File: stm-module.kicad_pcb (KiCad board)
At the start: 2 copper layers, 39.3 x 56.1 mm, 25 parts, among them J1 Conn_01x05_Pin, J2 connectorL, J3 connectorR, J4 power, SW1 Reset, U1 STM32G474RETx, U2 TPS7A20xxxDBV, Y1 Crystal

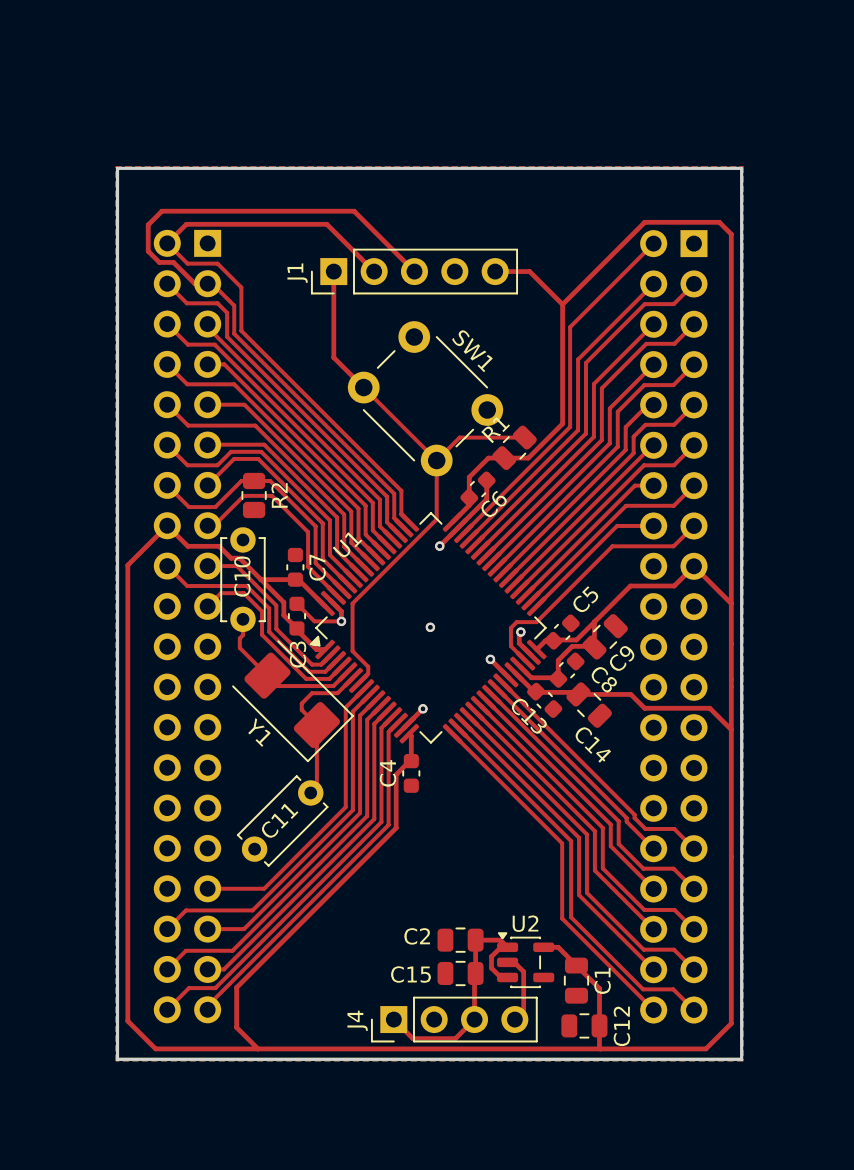
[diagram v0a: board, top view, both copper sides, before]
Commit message: more pcb updates
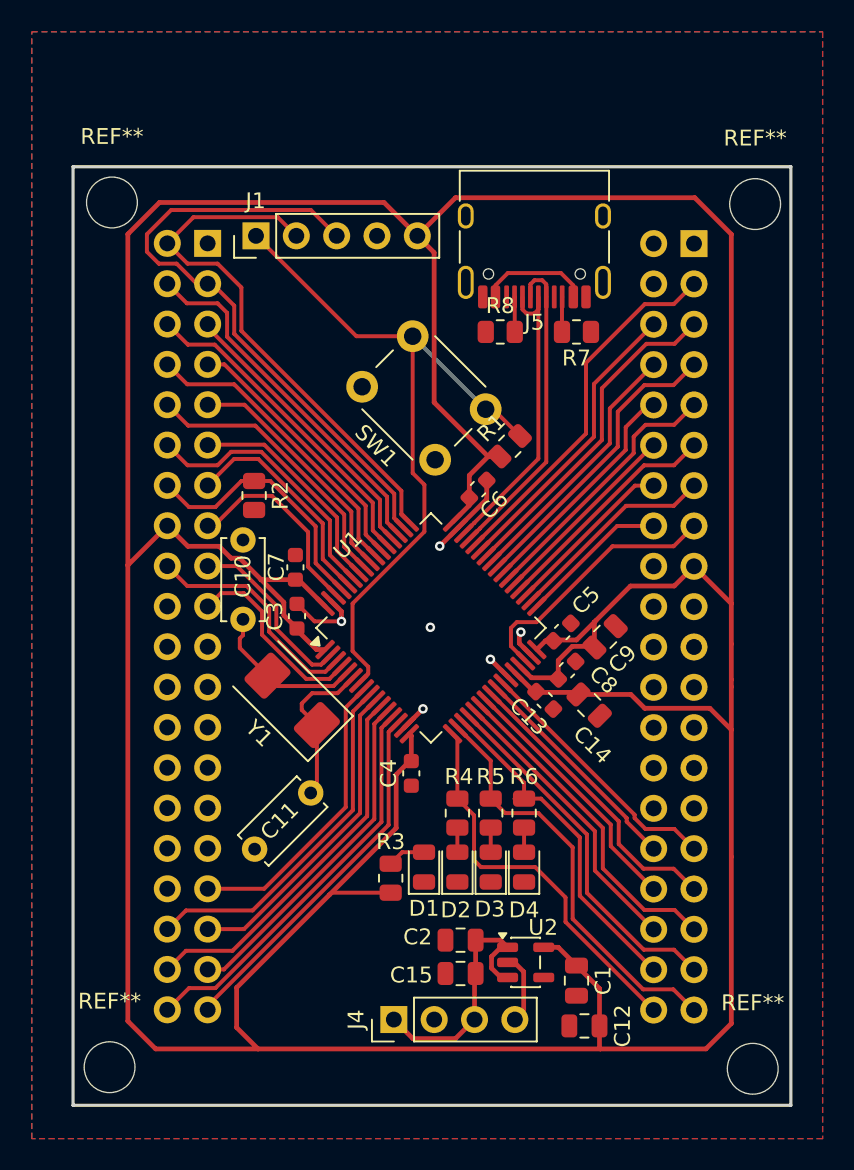
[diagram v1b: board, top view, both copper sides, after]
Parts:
- added D1: PWR LED, LED_SMD:LED_0805_2012Metric, F.Cu at (176.0, 141.1)
- added D2: RUN LED, LED_SMD:LED_0805_2012Metric, F.Cu at (178.1, 141.1)
- added D3: CAN LED, LED_SMD:LED_0805_2012Metric, F.Cu at (180.2, 141.1)
- added D4: FAULT LED, LED_SMD:LED_0805_2012Metric, F.Cu at (182.3, 141.1)
- added J5: USB_C_Receptacle_USB2.0_16P, Connector_USB:USB_C_Receptacle_HRO_TYPE-C-31-M-12, F.Cu at (182.9, 101.2)
- added R3: 330Ω, Resistor_SMD:R_0805_2012Metric, F.Cu at (173.9, 141.8)
- added R4: 220Ω, Resistor_SMD:R_0805_2012Metric, F.Cu at (178.1, 137.7)
- added R5: 1kΩ, Resistor_SMD:R_0805_2012Metric, F.Cu at (180.2, 137.7)
- added R6: 1kΩ, Resistor_SMD:R_0805_2012Metric, F.Cu at (182.3, 137.7)
- added R7: 5.1kΩ, Resistor_SMD:R_0805_2012Metric, F.Cu at (185.6, 107.4)
- added R8: 5.1kΩ, Resistor_SMD:R_0805_2012Metric, F.Cu at (180.8, 107.4)
- added REF**: MountingHole_3.2mm_M3, MountingHole:MountingHole_3.2mm_M3, F.Cu at (196.8, 99.3)
- added REF**: MountingHole_3.2mm_M3, MountingHole:MountingHole_3.2mm_M3, F.Cu at (196.7, 153.8)
- added REF**: MountingHole_3.2mm_M3, MountingHole:MountingHole_3.2mm_M3, F.Cu at (156.3, 99.2)
- added REF**: MountingHole_3.2mm_M3, MountingHole:MountingHole_3.2mm_M3, F.Cu at (156.2, 153.7)
- moved SW1 7.84 mm to (176.7, 115.5), turned to 135 degrees
- moved J1 5.39 mm to (165.4, 101.3)
- moved R1 0.32 mm to (181.4, 114.6)
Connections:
- J2 pad 20: unconnected-(J2-Pin_20-Pad20) -> GND
- J3 pad 2: /PA12 -> unconnected-(J3-Pin_2-Pad2)
- J3 pad 4: /PA11 -> unconnected-(J3-Pin_4-Pad4)
- U1 pad 45: /PA11 -> /D-
- U1 pad 46: /PA12 -> /D+
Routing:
- net +3.3V: track 248.2 -> 299.9 mm
- net /PA12: track 23.2 -> 0.00 mm
- net /PA11: track 20.9 -> 0.00 mm
- net /D-: track 0.00 -> 20.0 mm
- net /D+: track 0.00 -> 19.6 mm
- net /NRST: track 37.6 -> 46.5 mm
- net Net-(J5-VBUS-PadA4): track 0.00 -> 6.99 mm
- net /PA14: track 45.6 -> 39.7 mm
- net /PA13: track 39.7 -> 34.3 mm
- net Net-(D1-A): track 0.00 -> 2.40 mm
- net Net-(J5-SBU1): track 0.00 -> 2.21 mm
- net Net-(J5-SBU2): track 0.00 -> 2.21 mm
- net /PA3: track 22.6 -> 24.6 mm
- net Net-(D4-A): track 0.00 -> 1.55 mm
- net Net-(D3-A): track 0.00 -> 1.55 mm
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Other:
- board size 39.3 x 56.1 mm -> 45.2 x 59.1 mm
